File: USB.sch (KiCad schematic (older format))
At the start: 2 parts, among them P4 USB_OTG

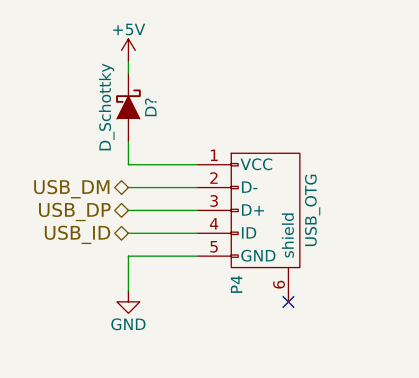
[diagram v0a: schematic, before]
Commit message: blubb
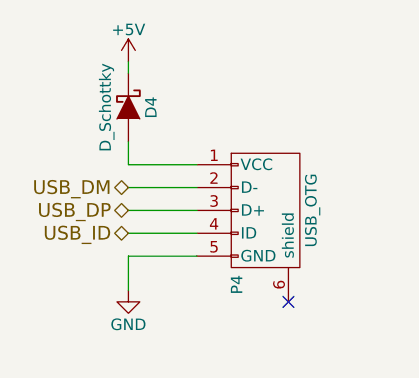
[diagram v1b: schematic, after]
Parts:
- D4: renamed from D?; footprint (none) -> Diodes_SMD:SOD-323
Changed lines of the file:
@@
 EESchema Schematic File Version 2
+LIBS:bldc-controller-rescue
 LIBS:power
 LIBS:device
@@
 LIBS:st-microelectronics
 LIBS:stm32
+LIBS:w_analog
+LIBS:mpu6000
 LIBS:bldc-controller-cache
 EELAYER 25 0
@@
 $Descr A4 11693 8268
 encoding utf-8
-Sheet 4 6
+Sheet 4 13
 Title "DreErolf"
 Date ""
@@
 $EndComp
 $Comp
-L +5V #PWR044
+L +5V #PWR023
 U 1 1 577D25D3
 P 1900 5350
-F 0 "#PWR044" H 1900 5200 50  0001 C CNN
+F 0 "#PWR023" H 1900 5200 50  0001 C CNN
 F 1 "+5V" H 1900 5490 50  0000 C CNN
 F 2 "" H 1900 5350 50  0000 C CNN
@@
 	1900 5800 2200 5800
 $Comp
-L GND #PWR045
+L GND #PWR024
 U 1 1 577D264D
 P 1900 6350
-F 0 "#PWR045" H 1900 6100 50  0001 C CNN
+F 0 "#PWR024" H 1900 6100 50  0001 C CNN
 F 1 "GND" H 1900 6200 50  0000 C CNN
 F 2 "" H 1900 6350 50  0000 C CNN
@@
 	2200 6100 1900 6100
 $Comp
-L D_Schottky D?
+L D_Schottky D4
 U 1 1 579031F5
 P 1900 5550
-F 0 "D?" H 1900 5650 50  0000 C CNN
+F 0 "D4" H 1900 5650 50  0000 C CNN
 F 1 "D_Schottky" H 1900 5450 50  0000 C CNN
-F 2 "" H 1900 5550 50  0000 C CNN
+F 2 "Diodes_SMD:SOD-323" H 1900 5550 50  0001 C CNN
 F 3 "" H 1900 5550 50  0000 C CNN
 	1    1900 5550

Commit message: routed
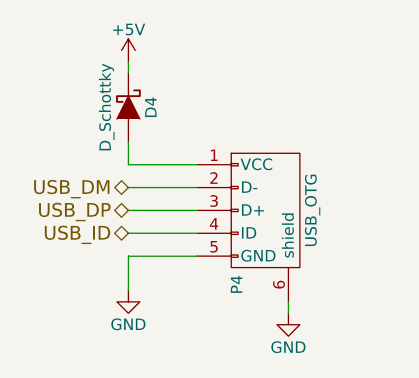
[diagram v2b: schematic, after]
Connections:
- net GND: now also P4.6 (shield)
- no-connect marks 1 -> 0
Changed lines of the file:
@@
 $Descr A4 11693 8268
 encoding utf-8
-Sheet 4 13
+Sheet 4 12
 Title "DreErolf"
 Date ""
@@
 $EndComp
 $Comp
-L +5V #PWR023
+L +5V #PWR022
 U 1 1 577D25D3
 P 1900 5350
-F 0 "#PWR023" H 1900 5200 50  0001 C CNN
+F 0 "#PWR022" H 1900 5200 50  0001 C CNN
 F 1 "+5V" H 1900 5490 50  0000 C CNN
 F 2 "" H 1900 5350 50  0000 C CNN
@@
 	1900 5800 2200 5800
 $Comp
-L GND #PWR024
+L GND #PWR023
 U 1 1 577D264D
 P 1900 6350
-F 0 "#PWR024" H 1900 6100 50  0001 C CNN
+F 0 "#PWR023" H 1900 6100 50  0001 C CNN
 F 1 "GND" H 1900 6200 50  0000 C CNN
 F 2 "" H 1900 6350 50  0000 C CNN
@@
 Wire Wire Line
 	1900 6200 1900 6350
-NoConn ~ 2600 6400
 Text HLabel 1900 6100 0    60   BiDi ~ 0
 USB_ID
@@
 	0    1    1    0
 $EndComp
+$Comp
+L GND #PWR?
+U 1 1 57B47666
+P 2600 6450
+F 0 "#PWR?" H 2600 6200 50  0001 C CNN
+F 1 "GND" H 2600 6300 50  0000 C CNN
+F 2 "" H 2600 6450 50  0000 C CNN
+F 3 "" H 2600 6450 50  0000 C CNN
+	1    2600 6450
+	1    0    0    -1
+$EndComp
+Wire Wire Line
+	2600 6450 2600 6400
 $EndSCHEMATC

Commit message: updated the part here
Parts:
- P4: symbol USB_OTG -> USB_OTG-RESCUE-bldc-controller
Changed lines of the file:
@@
 $EndDescr
 $Comp
-L USB_OTG P4
+L USB_OTG-RESCUE-bldc-controller P4
 U 1 1 577D256E
 P 2500 6000
+AR Path="/577D256E" Ref="P4"  Part="1"
+AR Path="/578E9D42/577D256E" Ref="P4"  Part="1"
 F 0 "P4" H 2825 5875 50  0000 C CNN
 F 1 "USB_OTG" H 2500 6200 50  0000 C CNN
